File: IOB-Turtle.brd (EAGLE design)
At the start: 20.3 x 50.8 mm, 22 parts, among them J1 RJ12/6, Q1 P-FET, Q2 P-FET, Q3 P-FET, Q4 P-FET

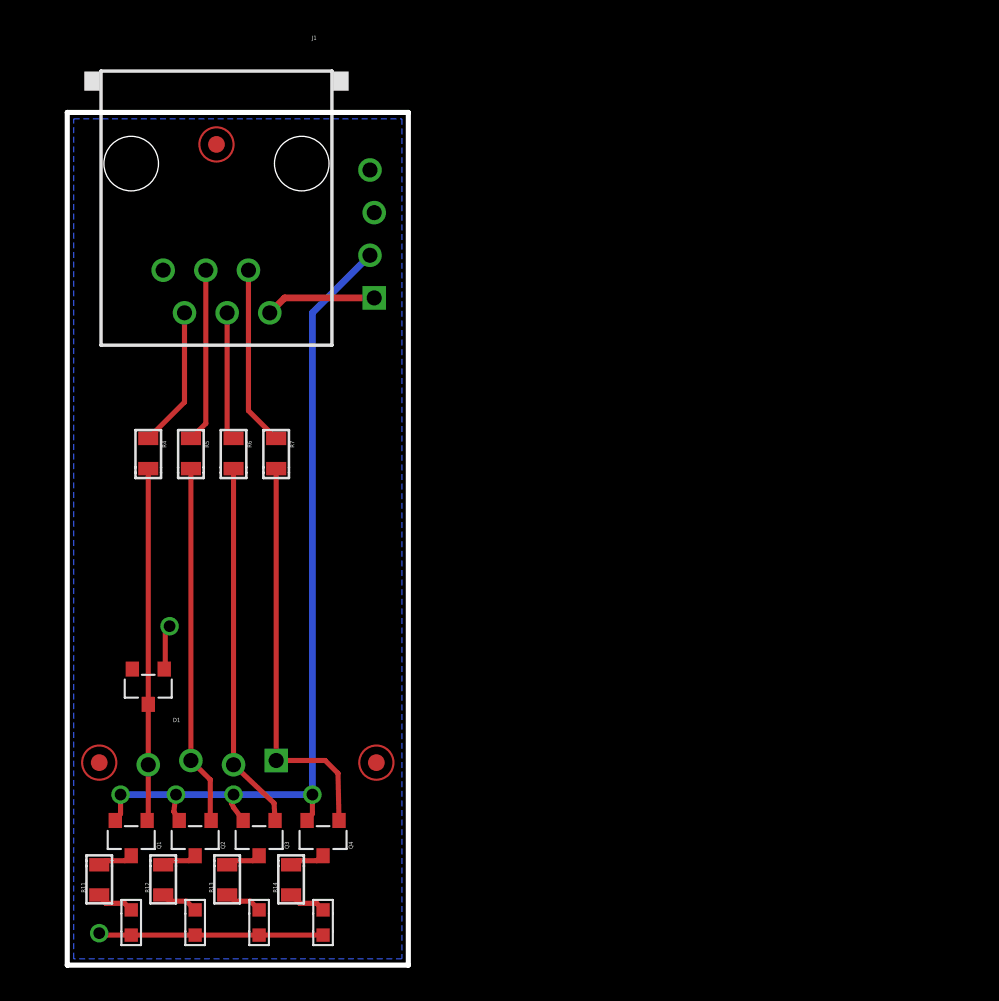
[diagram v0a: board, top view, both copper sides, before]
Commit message: Version 2.0
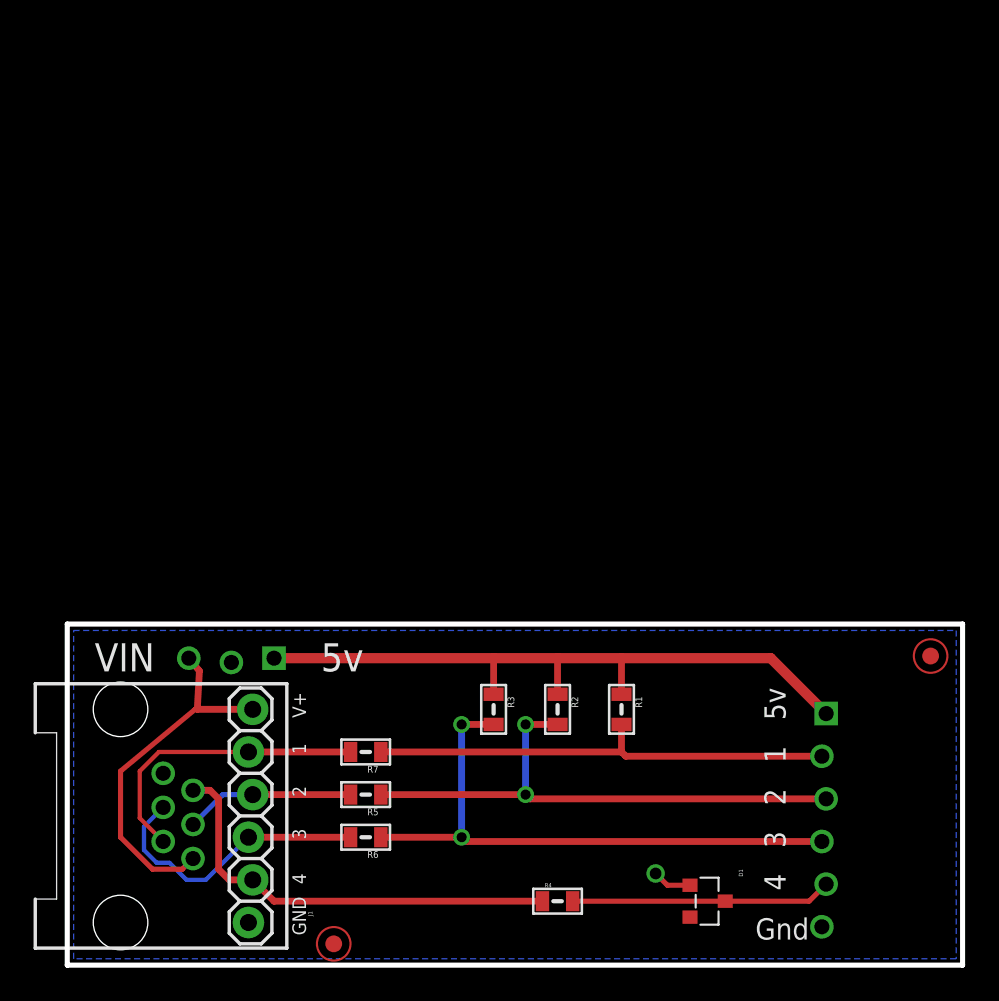
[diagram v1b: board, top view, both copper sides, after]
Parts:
- removed FID3: FIDUCIAL, SPCoast:FIDUCIAL_1MM
- removed IOB: IO4-IOBBARE, SPCoast:IO4-IOB
- removed LED1, LED3: G, SPCoast:0603-LED
- removed LED2: Y, SPCoast:0603-LED
- removed LED4: R, SPCoast:0603-LED
- removed Q1, Q2, Q3, Q4: P-FET, SPCoast:SOT23-3
- removed R11, R12, R13, R14: 2k0, SPCoast:0805-RES
- added R1, R2, R3: 10k, SPCoast:0805-RES
- added U$1: CONNECTOR-IO4-IOBBARE, SPCoast:IO4-IOB
- J1: device SPCoast:RJ25 -> SPCoast:RJ24-INVERTED-PINS
- R5, R6, R7: value 1k0 -> 200R
- moved FID2 49.9 mm to (51.4, 18.4), turned to 0 degrees
- moved FID1 48.1 mm to (15.9, 1.27), turned to 0 degrees
- moved J1 38.9 mm to (6.99, 8.89), turned to 90 degrees
- moved R4 36.1 mm to (29.2, 3.81), turned to 0 degrees
- moved D1 35.7 mm to (38.1, 3.81), turned to 270 degrees
- moved R6 24.2 mm to (17.8, 7.62), turned to 180 degrees
- moved R5 22.8 mm to (17.8, 10.2), turned to 180 degrees
- moved R7 18.6 mm to (17.8, 12.7), turned to 180 degrees
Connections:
- removed net !KT: J1.5, R4.1
- removed net N$11: Q4.3, R14.2
- removed net N$2: LED4.A, R14.1
- removed net N$3: LED3.A, R13.1
- removed net N$30: Q3.3, R13.2
- removed net N$31: Q2.3, R12.2
- removed net N$32: Q1.3, R11.2
- removed net N$4: LED2.A, R12.1
- removed net N$5: LED1.A, R11.1
- removed net P1: IOB.P1, Q4.1, R7.2
- removed net P2: IOB.P2, Q3.1, R6.2
- removed net P3: IOB.P3, Q2.1, R5.2
- new net IO4-2: J1.2, J1.2@1, R7.2
- new net IO4-3: J1.3, J1.3@1, R5.2
- new net IO4-4: J1.4, J1.4@1, R6.2
- new net IO4-5: J1.5, J1.5@1, R4.1
- net !NORM: now also R2.2, R5.1, U$1.P2; no longer J1.3, R6.1
- net !OCC: now also R3.2, R6.1, U$1.P3; no longer J1.4, R5.1
- net !REV: now also R1.2, U$1.P1; no longer J1.2
- net GND: now also J1.6@1, U$1.G@3; no longer IOB.G@1, IOB.G@2, LED1.C, LED2.C, LED3.C, LED4.C
- net P4: now also U$1.P4; no longer IOB.P4, Q1.1
- net VCC: now also R1.1, R2.1, R3.1, U$1.V5, U$1.V5@1; no longer IOB.V5, Q1.2, Q2.2, Q3.2, Q4.2
- net VCCIO: now also J1.1@1, U$1.V+; no longer IOB.V+
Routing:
- net IO4-5: track 0.00 -> 26.0 mm
- net !NORM: track 7.64 -> 32.7 mm, vias 0 -> 2
- net !OCC: track 10.4 -> 35.0 mm, vias 0 -> 2
- net P1: track 24.2 -> 0.00 mm
- net P2: track 22.0 -> 0.00 mm
- net P3: track 21.5 -> 0.00 mm
- net IO4-2: track 0.00 -> 17.8 mm
- net !REV: track 10.7 -> 28.0 mm
- net IO4-4: track 0.00 -> 17.1 mm
- net VCCIO: track 6.59 -> 21.8 mm
- net GND: track 16.1 -> 2.34 mm, vias 2 -> 1
- net VCC: track 51.7 -> 40.7 mm, vias 4 -> 0
- net IO4-3: track 0.00 -> 10.1 mm
- net !KT: track 8.38 -> 0.00 mm
- net P4: track 20.8 -> 15.5 mm
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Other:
- board size 20.3 x 50.8 mm -> 53.3 x 20.3 mm
- board text added: "2020-03"
- board text added: "D1"
- board text added: "Green Soldermask White Silkscreen"
- board text added: "J1"
- board text added: "R1"
- board text added: "R2"
- board text added: "R3"
- board text added: "R4"
- board text added: "R5"
- board text added: "R6"
- board text added: "R7"
- board text added: "v2.0"
- board text removed: "2018-02"
- board text removed: "IO Interface"
- board text removed: "Made in the PCR, Coast Div, NMRA"
- board text removed: "Model Railroading is Fun!"
- board text removed: "v1.1"
